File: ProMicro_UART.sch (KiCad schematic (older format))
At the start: 55 parts, among them J2 Conn_01x06, J3 USB_B_Mini, U1 FT232H, U2 93CxxB, U3 AZ1117-3.3, Y1 12Mhz

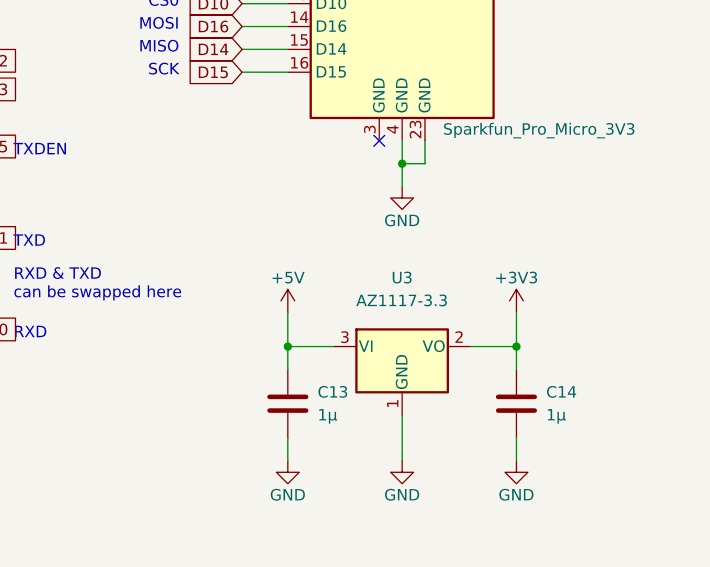
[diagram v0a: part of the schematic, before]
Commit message: new docs
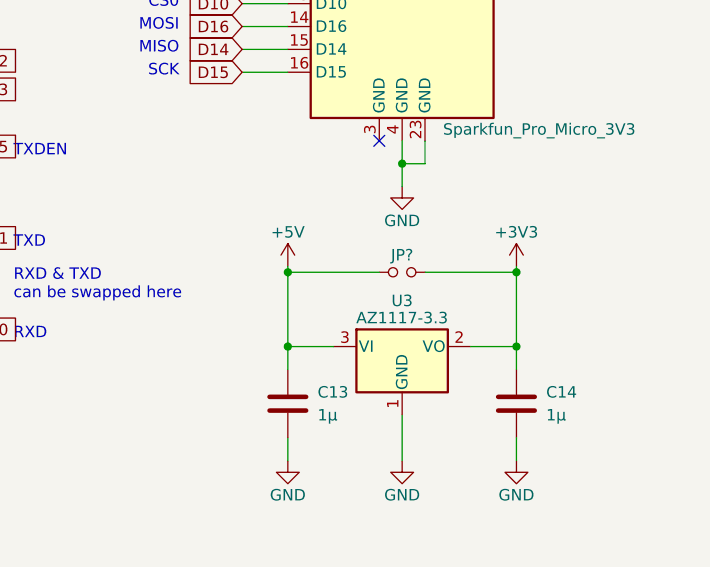
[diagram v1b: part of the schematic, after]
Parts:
- added JP?: Jumper_NO_Small, symbol Device:Jumper_NO_Small
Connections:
- net +3V3: now also JP?.2
- net +5V: now also JP?.1
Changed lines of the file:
@@
 U 1 1 5EE683B5
 P 9750 5500
-F 0 "U3" H 9750 5800 50  0000 C CNN
-F 1 "AZ1117-3.3" H 9750 5700 50  0000 C CNN
+F 0 "U3" H 9750 5700 50  0000 C CNN
+F 1 "AZ1117-3.3" H 9750 5625 50  0000 C CNN
 F 2 "Package_TO_SOT_SMD:SOT-23-5" H 9750 5750 50  0001 C CIN
 F 3 "https://www.diodes.com/assets/Datasheets/AZ1117.pdf" H 9750 5500 50  0001 C CNN
@@
 L power:+5V #PWR0135
 U 1 1 5EE78093
-P 9250 5350
-F 0 "#PWR0135" H 9250 5200 50  0001 C CNN
-F 1 "+5V" H 9250 5500 50  0000 C CNN
-F 2 "" H 9250 5350 50  0001 C CNN
-F 3 "" H 9250 5350 50  0001 C CNN
-	1    9250 5350
+P 9250 5150
+F 0 "#PWR0135" H 9250 5000 50  0001 C CNN
+F 1 "+5V" H 9250 5300 50  0000 C CNN
+F 2 "" H 9250 5150 50  0001 C CNN
+F 3 "" H 9250 5150 50  0001 C CNN
+	1    9250 5150
 	1    0    0    -1
 $EndComp
@@
 L power:+3V3 #PWR0136
 U 1 1 5EE7895F
-P 10250 5350
-F 0 "#PWR0136" H 10250 5200 50  0001 C CNN
-F 1 "+3V3" H 10250 5500 50  0000 C CNN
-F 2 "" H 10250 5350 50  0001 C CNN
-F 3 "" H 10250 5350 50  0001 C CNN
-	1    10250 5350
+P 10250 5150
+F 0 "#PWR0136" H 10250 5000 50  0001 C CNN
+F 1 "+3V3" H 10250 5300 50  0000 C CNN
+F 2 "" H 10250 5150 50  0001 C CNN
+F 3 "" H 10250 5150 50  0001 C CNN
+	1    10250 5150
 	1    0    0    -1
 $EndComp
@@
 Connection ~ 9250 5500
 Wire Wire Line
-	9250 5500 9250 5350
+	9250 5500 9250 5175
 Wire Wire Line
 	10050 5500 10250 5500
 Wire Wire Line
-	10250 5500 10250 5350
+	10250 5500 10250 5175
 Wire Wire Line
 	10250 5600 10250 5500
@@
 Wire Wire Line
 	6750 3875 6750 4625
+$Comp
+L Device:Jumper_NO_Small JP?
+U 1 1 5E6685A0
+P 9750 5175
+F 0 "JP?" H 9750 5250 50  0000 C CNN
+F 1 "Jumper_NO_Small" H 9775 5275 50  0001 C CNN
+F 2 "" H 9750 5175 50  0001 C CNN
+F 3 "~" H 9750 5175 50  0001 C CNN
+	1    9750 5175
+	1    0    0    -1
+$EndComp
+Wire Wire Line
+	9850 5175 10250 5175
+Connection ~ 10250 5175
+Wire Wire Line
+	10250 5175 10250 5150
+Wire Wire Line
+	9650 5175 9250 5175
+Connection ~ 9250 5175
+Wire Wire Line
+	9250 5175 9250 5150
 $EndSCHEMATC
